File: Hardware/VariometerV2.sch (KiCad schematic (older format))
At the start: 107 parts, among them IC1 TP4056, IC2 DW01A-G, IC3 ESP32-S3-WROOM-1, J1 LED_CHRG, J2 LED_STBY, J3 TFT_LCD_CONNECTOR, J4 Conn_01x02_Male, J5 SWD, J6 USB3135-30-A, J7 5-1814832-1, J8 Conn_02x01, J9 MEM2075-00-140-01-A, Q1 AO3400A, Q10 AO3400A, Q2 AO3400A, Q3 AO3401A, Q4 AO3400A, Q5 AO3401A, Q6 AO3400A, Q7 AO3401A, Q8 AO3400A, Q9 AO3401A, SW1 SW_Push, SW2 Switch_SW_Push, SW3 Switch_SW_Push, SW4 SW_Push, U1 TPS76801QDR, U2 SRV05-4, U4 ATGM336H-5N31, U5 SRV05-4, U6 SRV05-4, U7 BMI088, U8 MS5611-01BA

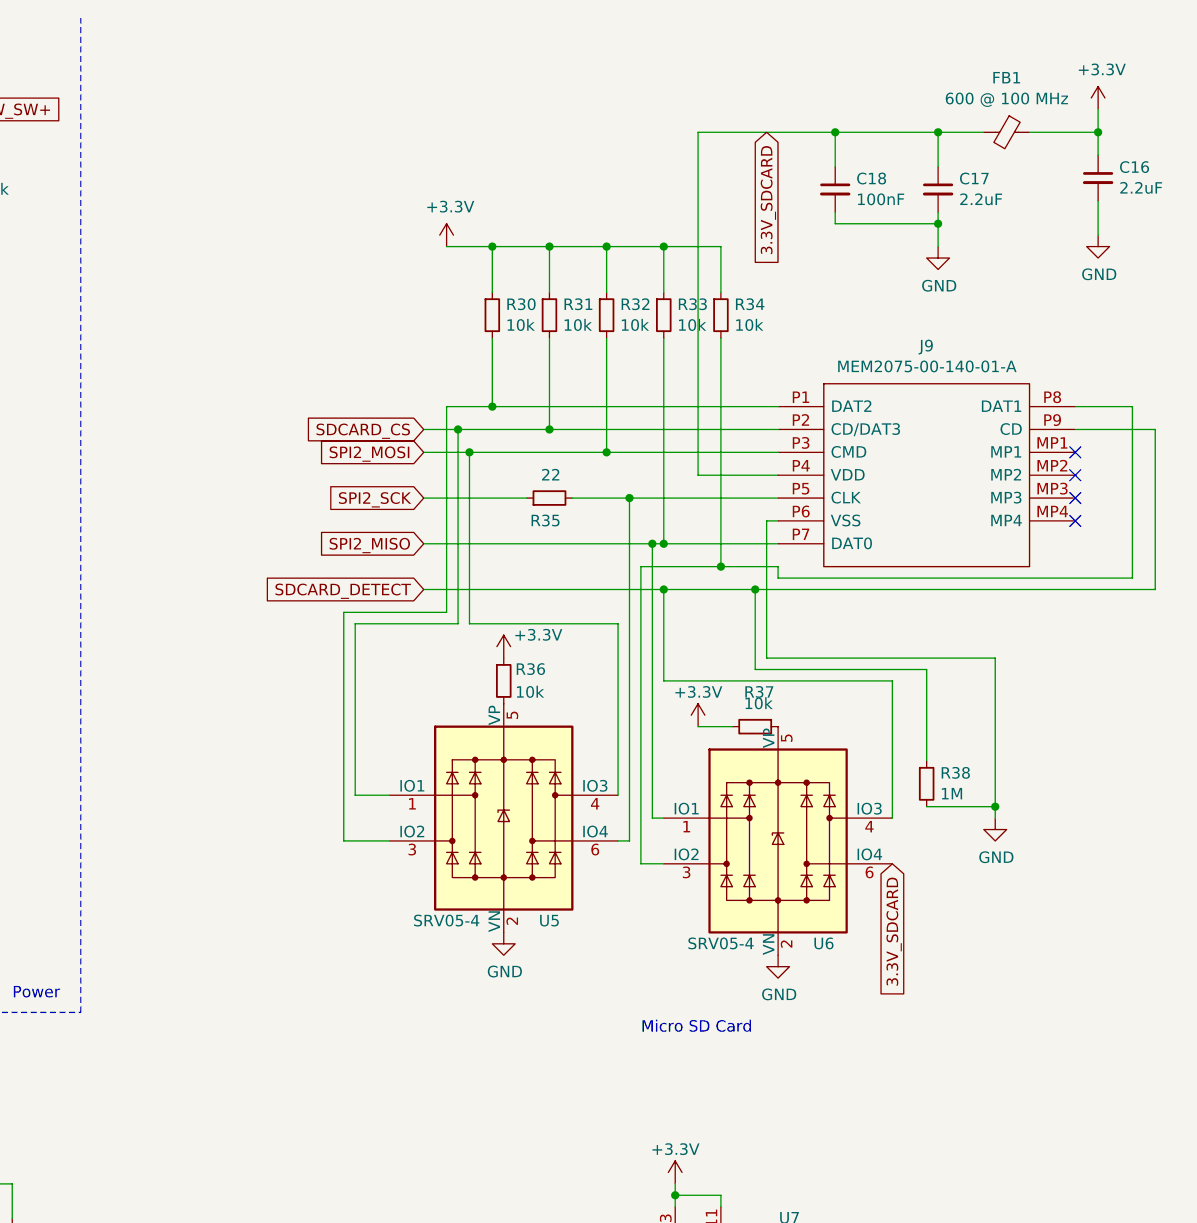
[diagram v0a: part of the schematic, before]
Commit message: update
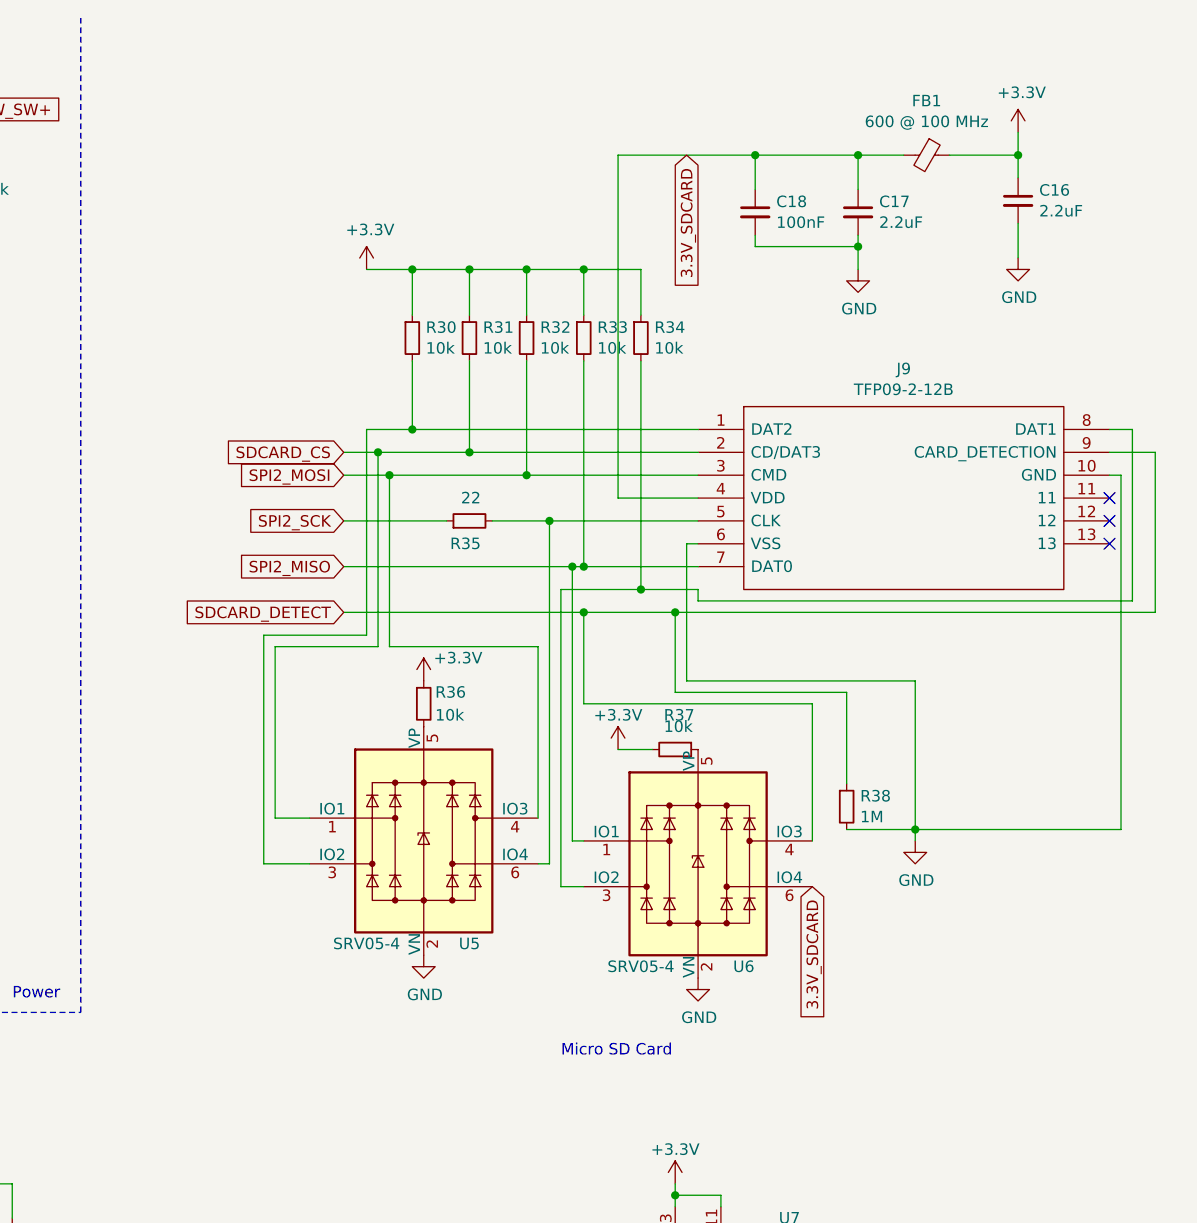
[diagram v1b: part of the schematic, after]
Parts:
- removed J9: MEM2075-00-140-01-A, Hardware:MEM20750014001A, symbol SamacSys_Parts:MEM2075-00-140-01-A
- added J9: TFP09-2-12B, Hardware:TFP09212B, symbol SamacSys_Parts:TFP09-2-12B
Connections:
- net 3.3V_SDCARD: now also J9.4 (VDD)
- net GND: now also J9.10 (GND), J9.6 (VSS)
- net SDCARD_CS: now also J9.2 (CD/DAT3)
- net SDCARD_DETECT: now also J9.9 (CARD_DETECTION)
- net SPI2_MISO: now also J9.7 (DAT0)
- net SPI2_MOSI: now also J9.3 (CMD)
- net at R30.2, U5.3 (IO2): now also J9.1 (DAT2)
- net at R35.2, U5.6 (IO4): now also J9.5 (CLK)
- net at R34.2, U6.3 (IO2): now also J9.8 (DAT1)
- no-connect marks 25 -> 24
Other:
- moved on the sheet: C16, C17, C18, FB1, R30, R31, R32, R33, R34, R35, R36, R37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
